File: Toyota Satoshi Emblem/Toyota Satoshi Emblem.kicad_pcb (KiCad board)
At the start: 2 copper layers, 175 x 151 mm, 366 parts

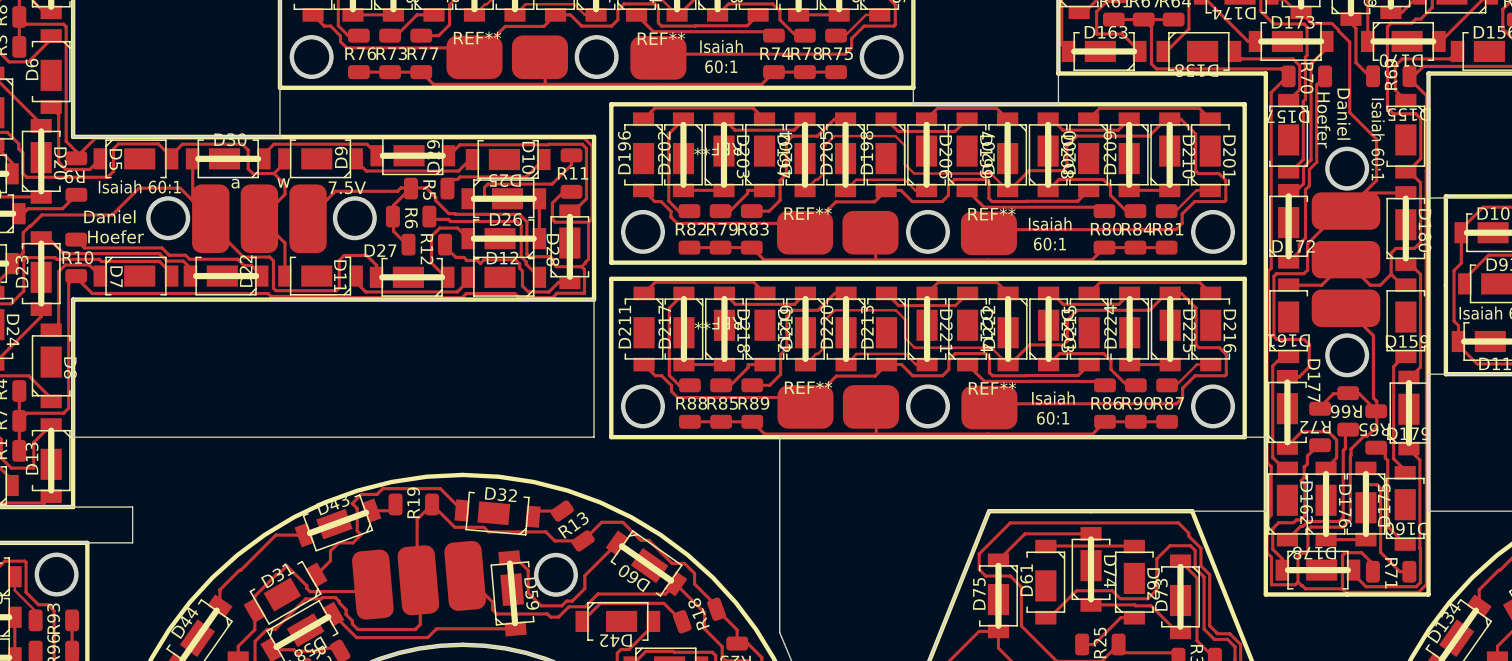
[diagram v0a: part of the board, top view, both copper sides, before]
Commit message: v1.13
Yet more schematic changes
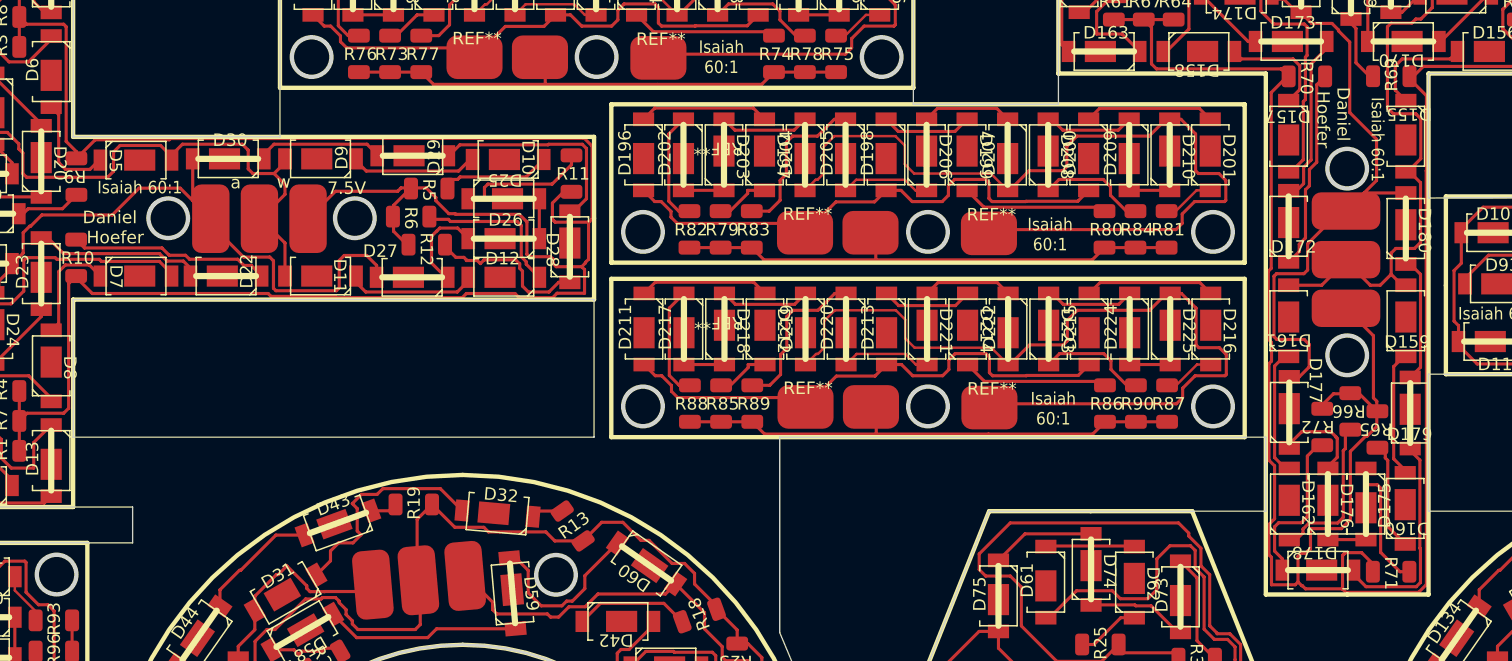
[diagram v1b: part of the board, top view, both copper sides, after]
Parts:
- moved R72 0.17 mm to (127.7, 203.9)
- moved R66 0.17 mm to (130.0, 202.6)
- moved D162 0.15 mm to (125.1, 210.1)
- moved D177 0.15 mm to (125.1, 202.7)
- moved D176 0.15 mm to (128.2, 210.1)
- moved D179 0.10 mm to (134.8, 202.8)
- moved D5 0.10 mm to (32.6, 182.5)
- moved R65 0.10 mm to (132.2, 204.1)
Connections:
- R79 pad 1: Net-(J19-Pad2) -> Net-(R79-Pad1)
- R80 pad 1: Net-(J19-Pad2) -> Net-(R79-Pad1)
- R81 pad 1: Net-(J19-Pad2) -> Net-(R79-Pad1)
- R82 pad 1: Net-(J19-Pad2) -> Net-(R79-Pad1)
- R83 pad 1: Net-(J19-Pad2) -> Net-(R79-Pad1)
- R84 pad 1: Net-(J19-Pad2) -> Net-(R79-Pad1)
- R85 pad 1: Net-(J20-Pad2) -> Net-(R85-Pad1)
- R86 pad 1: Net-(J20-Pad2) -> Net-(R85-Pad1)
- R87 pad 1: Net-(J20-Pad2) -> Net-(R85-Pad1)
- R88 pad 1: Net-(J20-Pad2) -> Net-(R85-Pad1)
- R89 pad 1: Net-(J20-Pad2) -> Net-(R85-Pad1)
- R90 pad 1: Net-(J20-Pad2) -> Net-(R85-Pad1)
- REF** pad 1: Net-(R91-Pad1) -> Net-(J21-Pad2)
- REF** pad 1: Net-(R61-Pad1) -> Net-(J10-Pad2)
- REF** pad 1: Net-(R76-Pad1) -> Net-(J17-Pad2)
- REF** pad 1: Net-(R82-Pad1) -> Net-(R79-Pad1)
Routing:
- net Net-(R79-Pad1): track 0.00 -> 41.5 mm
- net Net-(J19-Pad2): track 41.5 -> 0.00 mm
- net Net-(R85-Pad1): track 0.00 -> 41.5 mm
- net Net-(J20-Pad2): track 41.5 -> 0.00 mm
- net Net-(D161-Pad2): track 11.8 -> 12.4 mm
